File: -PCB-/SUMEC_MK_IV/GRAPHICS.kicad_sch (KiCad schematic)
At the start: 4 parts

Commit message: v3.0.9 SUMEC PCB
Ufff, so, basically a full rewrite of the PCB, check it our its pretty sick, I think
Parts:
- renumbered R27 to R20, R28 to R21, R29 to R22, R30 to R23
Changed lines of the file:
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@@
 	(title_block
 		(title "SUMEC_MK_IV")
-		(date "2024-07-15")
-		(rev "v3.0.0")
+		(date "2024-08-05")
+		(rev "v3.0.9")
 		(company "SPS NA PROSEKU")
 		(comment 1 "Made in Prague, Czech Republic")
@@
 		(dnp no)
 		(fields_autoplaced yes)
-		(property "Reference" "R27"
+		(property "Reference" "R20"
 			(at 147.32 83.82 90)
 			(effects
@@
 			(project "SUMEC_MK_IV"
 				(path "/900bd7ac-cdf9-4a2f-8b1f-2c21e3760046/ebfdffb9-be38-48cc-bdc4-81d227bad184"
-					(reference "R27")
+					(reference "R20")
 					(unit 1)
 				)
@@
 		(dnp no)
 		(fields_autoplaced yes)
-		(property "Reference" "R28"
+		(property "Reference" "R21"
 			(at 147.32 90.17 90)
 			(effects
@@
 			(project "SUMEC_MK_IV"
 				(path "/900bd7ac-cdf9-4a2f-8b1f-2c21e3760046/ebfdffb9-be38-48cc-bdc4-81d227bad184"
-					(reference "R28")
+					(reference "R21")
 					(unit 1)
 				)
@@
 		(dnp no)
 		(fields_autoplaced yes)
-		(property "Reference" "R29"
+		(property "Reference" "R22"
 			(at 147.32 96.52 90)
 			(effects
@@
 			(project "SUMEC_MK_IV"
 				(path "/900bd7ac-cdf9-4a2f-8b1f-2c21e3760046/ebfdffb9-be38-48cc-bdc4-81d227bad184"
-					(reference "R29")
+					(reference "R22")
 					(unit 1)
 				)
@@
 		(dnp no)
 		(fields_autoplaced yes)
-		(property "Reference" "R30"
+		(property "Reference" "R23"
 			(at 147.32 102.87 90)
 			(effects
@@
 			(project "SUMEC_MK_IV"
 				(path "/900bd7ac-cdf9-4a2f-8b1f-2c21e3760046/ebfdffb9-be38-48cc-bdc4-81d227bad184"
-					(reference "R30")
+					(reference "R23")
 					(unit 1)
 				)

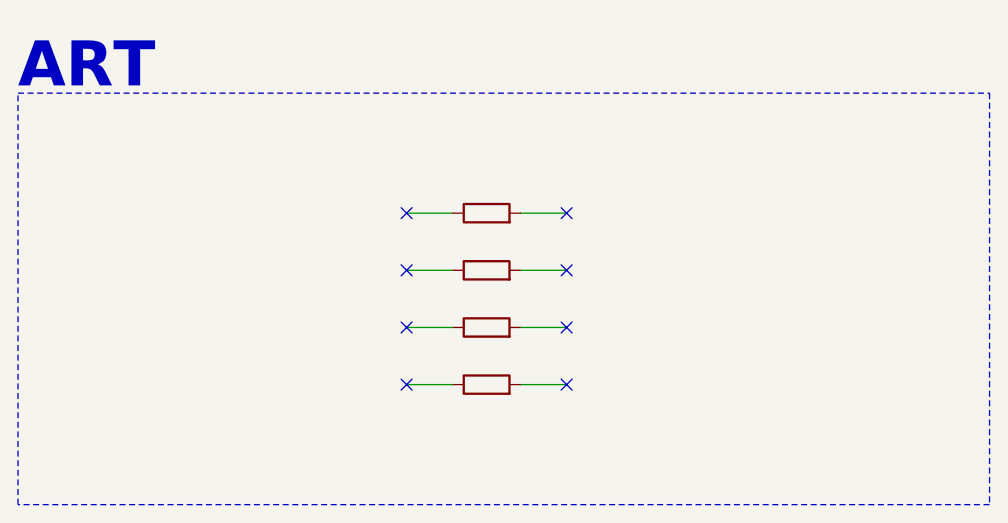
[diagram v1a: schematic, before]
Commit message: DRC Hell fix
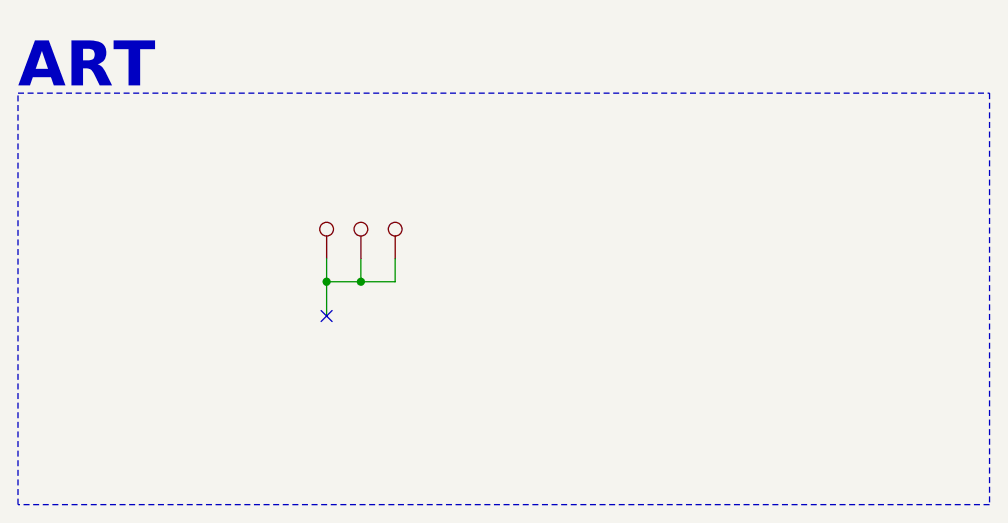
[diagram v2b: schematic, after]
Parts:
- removed R20: R, sumec-remote_library:purosidenegative, symbol Device:R
- removed R21: R, sumec-smdV2_library:SPS LOGO, symbol Device:R
- removed R22: R, sumec-remote_library:boi, symbol Device:R
- removed R23: R, sumec-smdV2_library:Logo, symbol Device:R
- added TP5: TestPoint, sumec_graphic:SPS_LOGO_IMG, symbol Connector:TestPoint
- added TP6: TestPoint, sumec_graphic:SUMEC_LOGO_IMG, symbol Connector:TestPoint
- added TP7: TestPoint, sumec_graphic:ULTRAKILL_IMG, symbol Connector:TestPoint
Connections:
- new net: TP5.1, TP6.1, TP7.1
- no-connect marks 8 -> 1
